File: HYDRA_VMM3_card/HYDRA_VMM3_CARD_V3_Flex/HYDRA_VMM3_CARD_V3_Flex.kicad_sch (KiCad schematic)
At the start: 22 parts, among them J1 ME1014010101011

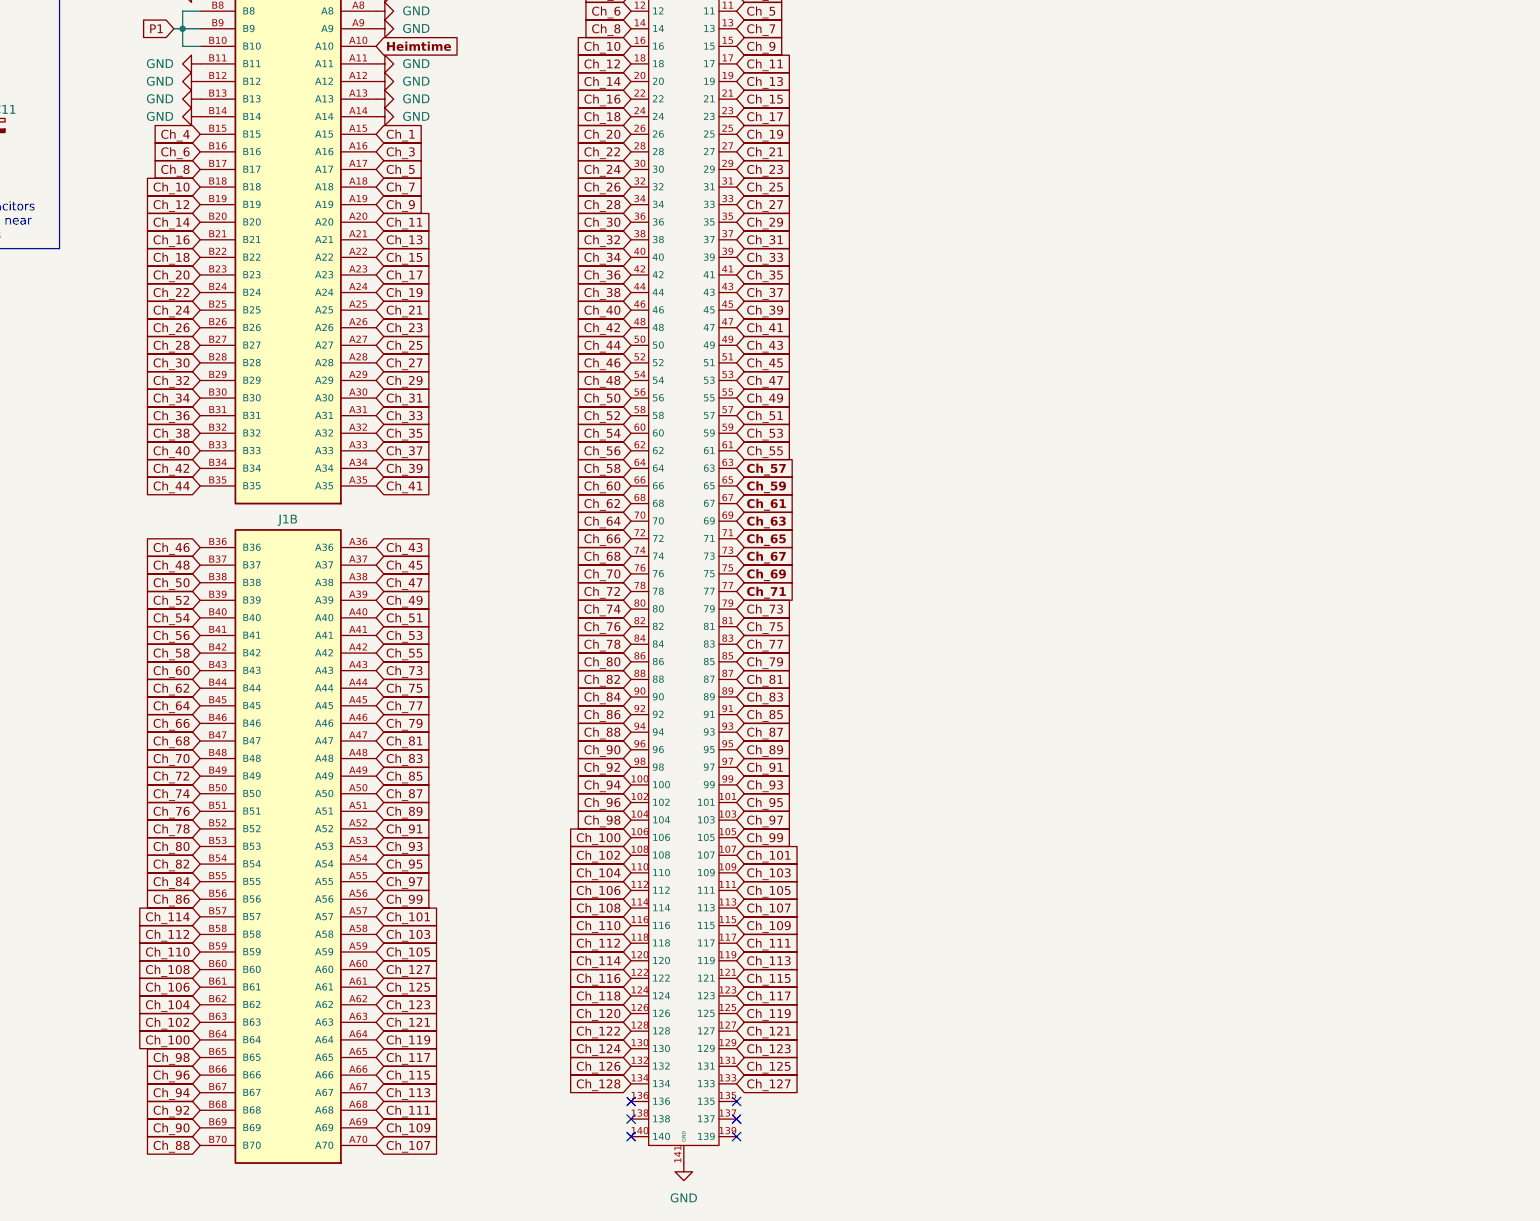
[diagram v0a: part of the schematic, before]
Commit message: .
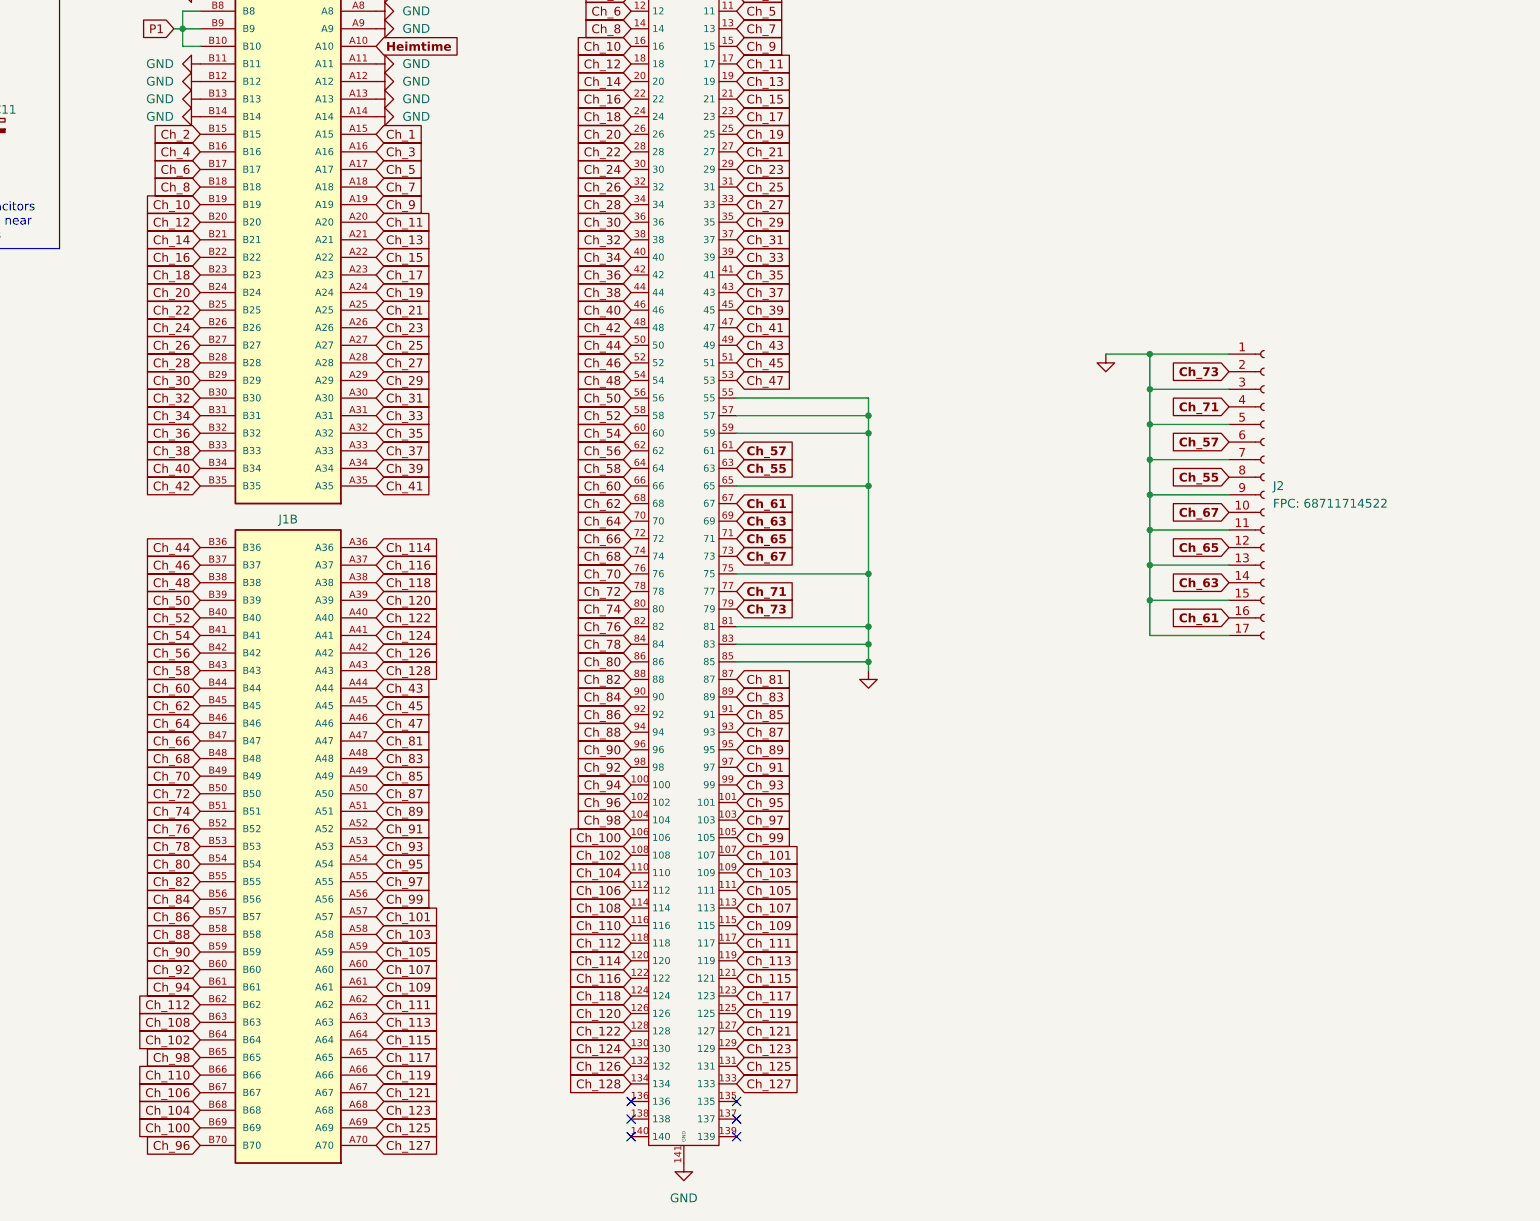
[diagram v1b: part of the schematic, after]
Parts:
- added J2: FPC: 68711714522, Custom_Footprints:68711714522, symbol Connector:Conn_01x17_Socket
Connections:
- net Ch_59 is gone; now on net GND: U1.65
- net Ch_69 is gone; now on net GND: U1.75
- net Ch_10: now also J1.B19; no longer J1.B18
- net Ch_100: now also J1.B69; no longer J1.B64
- net Ch_102: now also J1.B64; no longer J1.B63
- net Ch_104: now also J1.B68; no longer J1.B62
- net Ch_106: now also J1.B67; no longer J1.B61
- net Ch_107: now also J1.A60; no longer J1.A70
- net Ch_108: now also J1.B63; no longer J1.B60
- net Ch_109: now also J1.A61; no longer J1.A69
- net Ch_110: now also J1.B66; no longer J1.B59
- net Ch_111: now also J1.A62; no longer J1.A68
- net Ch_112: now also J1.B62; no longer J1.B58
- net Ch_113: now also J1.A63; no longer J1.A67
- net Ch_114: now also J1.A36; no longer J1.B57
- net Ch_115: now also J1.A64; no longer J1.A66
- net Ch_116: now also J1.A37
- net Ch_118: now also J1.A38
- net Ch_119: now also J1.A66; no longer J1.A64
- net Ch_12: now also J1.B20; no longer J1.B19
- net Ch_120: now also J1.A39
- net Ch_121: now also J1.A67; no longer J1.A63
- net Ch_122: now also J1.A40
- net Ch_123: now also J1.A68; no longer J1.A62
- net Ch_124: now also J1.A41
- net Ch_125: now also J1.A69; no longer J1.A61
- net Ch_126: now also J1.A42
- net Ch_127: now also J1.A70; no longer J1.A60
- net Ch_128: now also J1.A43
- net Ch_14: now also J1.B21; no longer J1.B20
- net Ch_16: now also J1.B22; no longer J1.B21
- net Ch_18: now also J1.B23; no longer J1.B22
- net Ch_2: now also J1.B15
- net Ch_20: now also J1.B24; no longer J1.B23
- net Ch_22: now also J1.B25; no longer J1.B24
- net Ch_24: now also J1.B26; no longer J1.B25
- net Ch_26: now also J1.B27; no longer J1.B26
- net Ch_28: now also J1.B28; no longer J1.B27
- net Ch_30: now also J1.B29; no longer J1.B28
- net Ch_32: now also J1.B30; no longer J1.B29
- net Ch_34: now also J1.B31; no longer J1.B30
- net Ch_36: now also J1.B32; no longer J1.B31
- net Ch_38: now also J1.B33; no longer J1.B32
- net Ch_4: now also J1.B16; no longer J1.B15
- net Ch_40: now also J1.B34; no longer J1.B33
- net Ch_42: now also J1.B35; no longer J1.B34
- net Ch_43: now also J1.A44; no longer J1.A36
- net Ch_44: now also J1.B36; no longer J1.B35
- net Ch_45: now also J1.A45; no longer J1.A37
- net Ch_46: now also J1.B37; no longer J1.B36
- net Ch_47: now also J1.A46; no longer J1.A38
- net Ch_48: now also J1.B38; no longer J1.B37
- net Ch_50: now also J1.B39; no longer J1.B38
- net Ch_52: now also J1.B40; no longer J1.B39
- net Ch_54: now also J1.B41; no longer J1.B40
- net Ch_55: now also U1.63, J2.8 (Pin_8); no longer J1.A42, U1.61
- net Ch_56: now also J1.B42; no longer J1.B41
- net Ch_57: now also U1.61, J2.6 (Pin_6); no longer U1.63
- net Ch_58: now also J1.B43; no longer J1.B42
- net Ch_6: now also J1.B17; no longer J1.B16
- net Ch_60: now also J1.B44; no longer J1.B43
- net Ch_61: now also J2.16 (Pin_16)
- net Ch_62: now also J1.B45; no longer J1.B44
- net Ch_63: now also J2.14 (Pin_14)
- net Ch_64: now also J1.B46; no longer J1.B45
- net Ch_65: now also J2.12 (Pin_12)
- net Ch_66: now also J1.B47; no longer J1.B46
- net Ch_67: now also J2.10 (Pin_10)
- net Ch_68: now also J1.B48; no longer J1.B47
- net Ch_70: now also J1.B49; no longer J1.B48
- net Ch_71: now also J2.4 (Pin_4)
- net Ch_72: now also J1.B50; no longer J1.B49
- net Ch_73: now also J2.2 (Pin_2); no longer J1.A43
- net Ch_74: now also J1.B51; no longer J1.B50
- net Ch_76: now also J1.B52; no longer J1.B51
- net Ch_78: now also J1.B53; no longer J1.B52
- net Ch_8: now also J1.B18; no longer J1.B17
- net Ch_80: now also J1.B54; no longer J1.B53
- net Ch_82: now also J1.B55; no longer J1.B54
- net Ch_84: now also J1.B56; no longer J1.B55
- net Ch_86: now also J1.B57; no longer J1.B56
- net Ch_88: now also J1.B58; no longer J1.B70
- net Ch_90: now also J1.B59; no longer J1.B69
- net Ch_92: now also J1.B60; no longer J1.B68
- net Ch_94: now also J1.B61; no longer J1.B67
- net Ch_96: now also J1.B70; no longer J1.B66
- net GND: now also U1.55, U1.57, U1.59, U1.81, U1.83, U1.85, J2.1 (Pin_1), J2.11 (Pin_11), J2.13 (Pin_13), J2.15 (Pin_15), J2.17 (Pin_17), J2.3 (Pin_3), J2.5 (Pin_5), J2.7 (Pin_7), J2.9 (Pin_9)
- removed net Ch_49: J1.A39, U1.55
- removed net Ch_51: J1.A40, U1.57
- removed net Ch_53: J1.A41, U1.59
- removed net Ch_75: J1.A44, U1.81
- removed net Ch_77: J1.A45, U1.83
- removed net Ch_79: J1.A46, U1.85

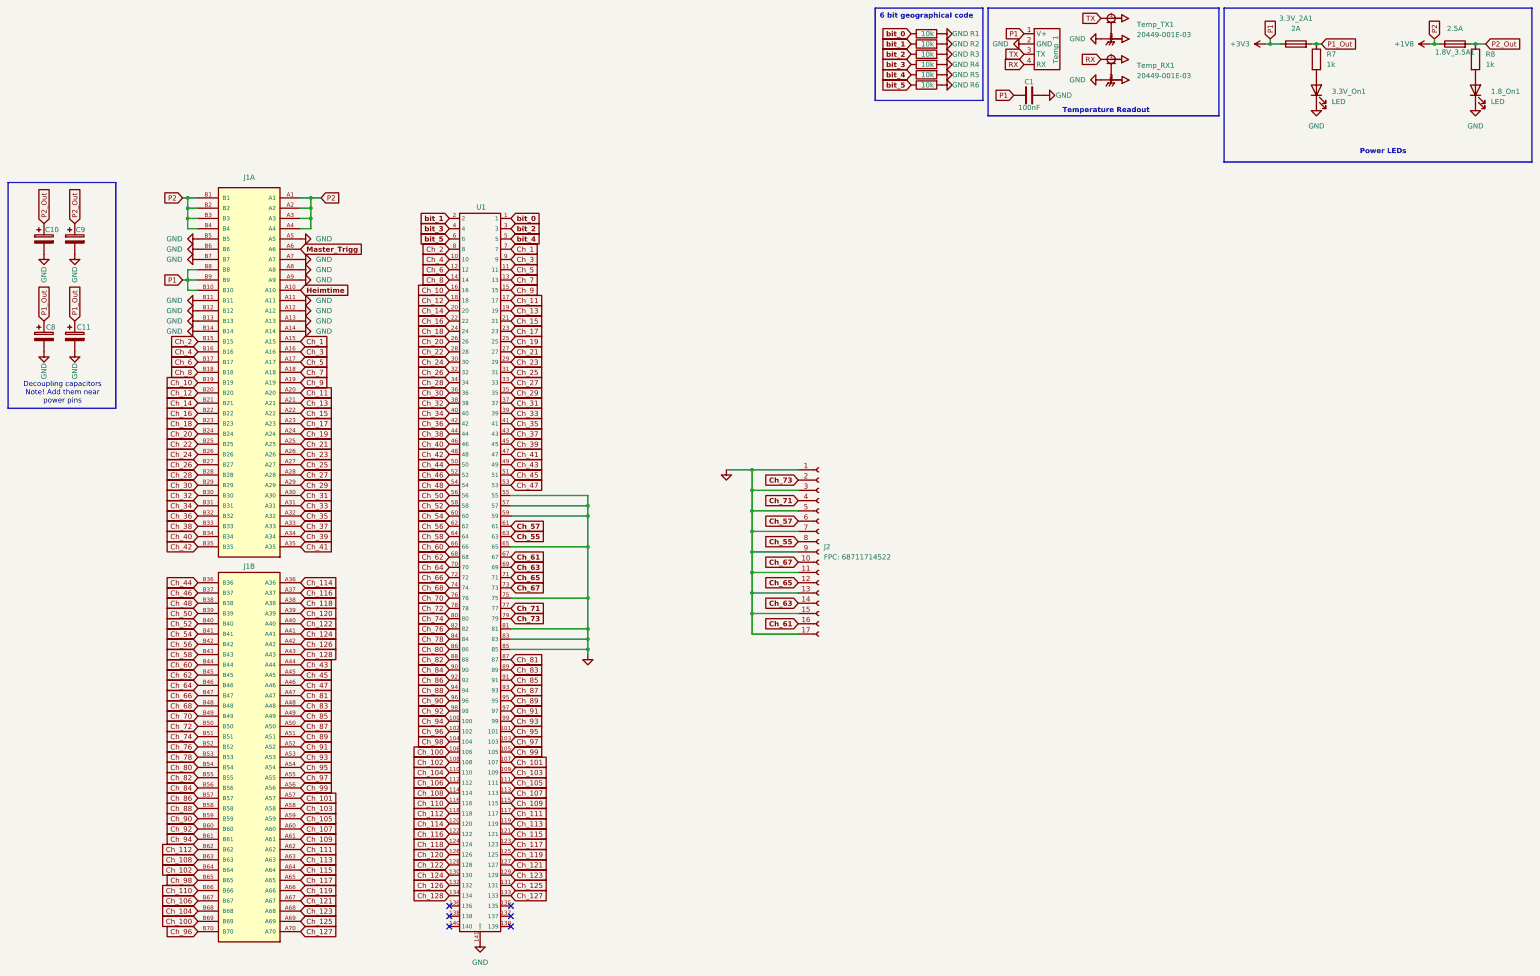
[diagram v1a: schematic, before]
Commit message: .
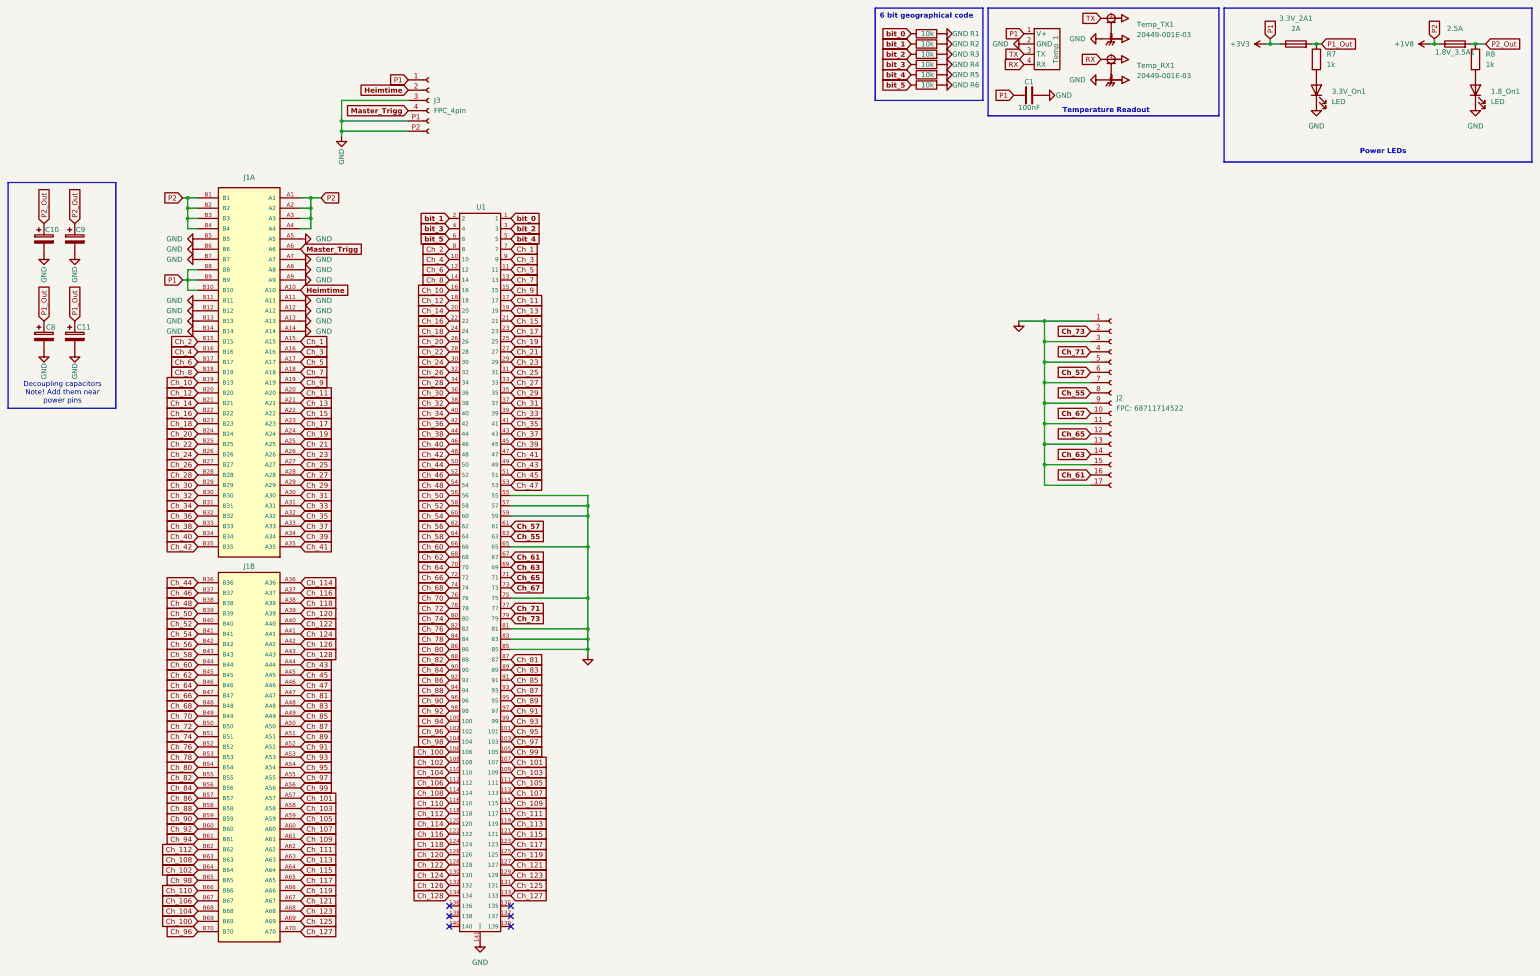
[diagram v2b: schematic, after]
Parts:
- added J3: FPC_4pin, Custom_Footprints:CON_5034800440_MOL, symbol Connector:Conn_01x06_Socket
- Temp_RX1, Temp_TX1: footprint IPEX:IPEX_20449-001E-03 -> Custom_Footprints:IPEX_20449-001E-03
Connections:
- net +3V3: now also J3.1 (Pin_1)
- net GND: now also J3.3 (Pin_3), J3.P1 (Pin_5), J3.P2 (Pin_6)
- net Heimtime: now also J3.2 (Pin_2)
- net Master_Trigg: now also J3.4 (Pin_4)
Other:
- moved on the sheet: J2
